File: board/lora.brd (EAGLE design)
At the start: 20.2 x 72.9 mm, 33 parts, among them IC1 STM32F030F4, IC2 ADP1607, J1 SWD_PTH_SHROUD, X1 SMA-142-0701-801/806, X2 UBLOX_MAX, X3 RFM98

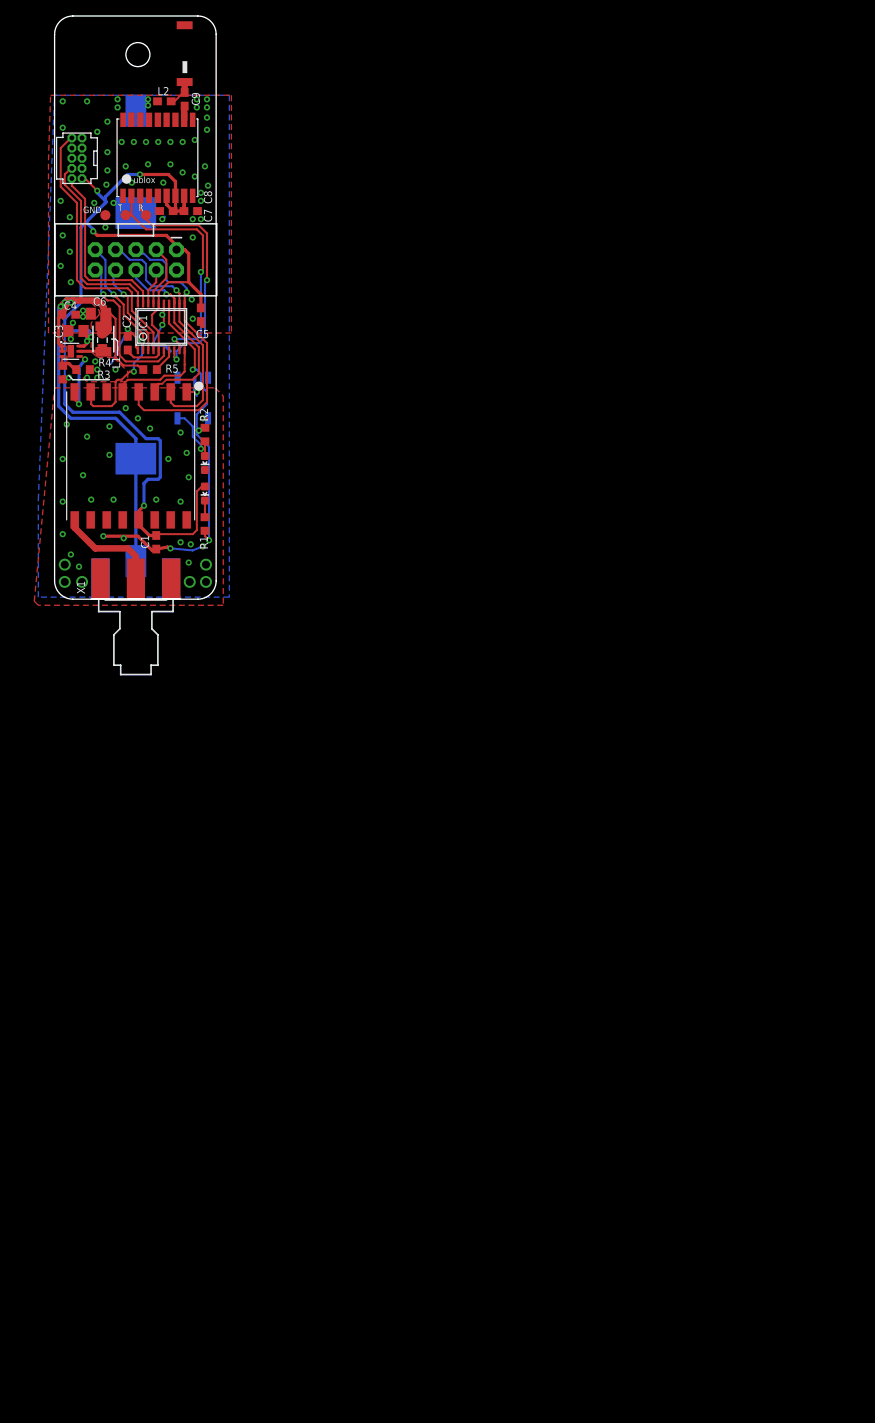
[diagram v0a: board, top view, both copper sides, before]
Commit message: improvments
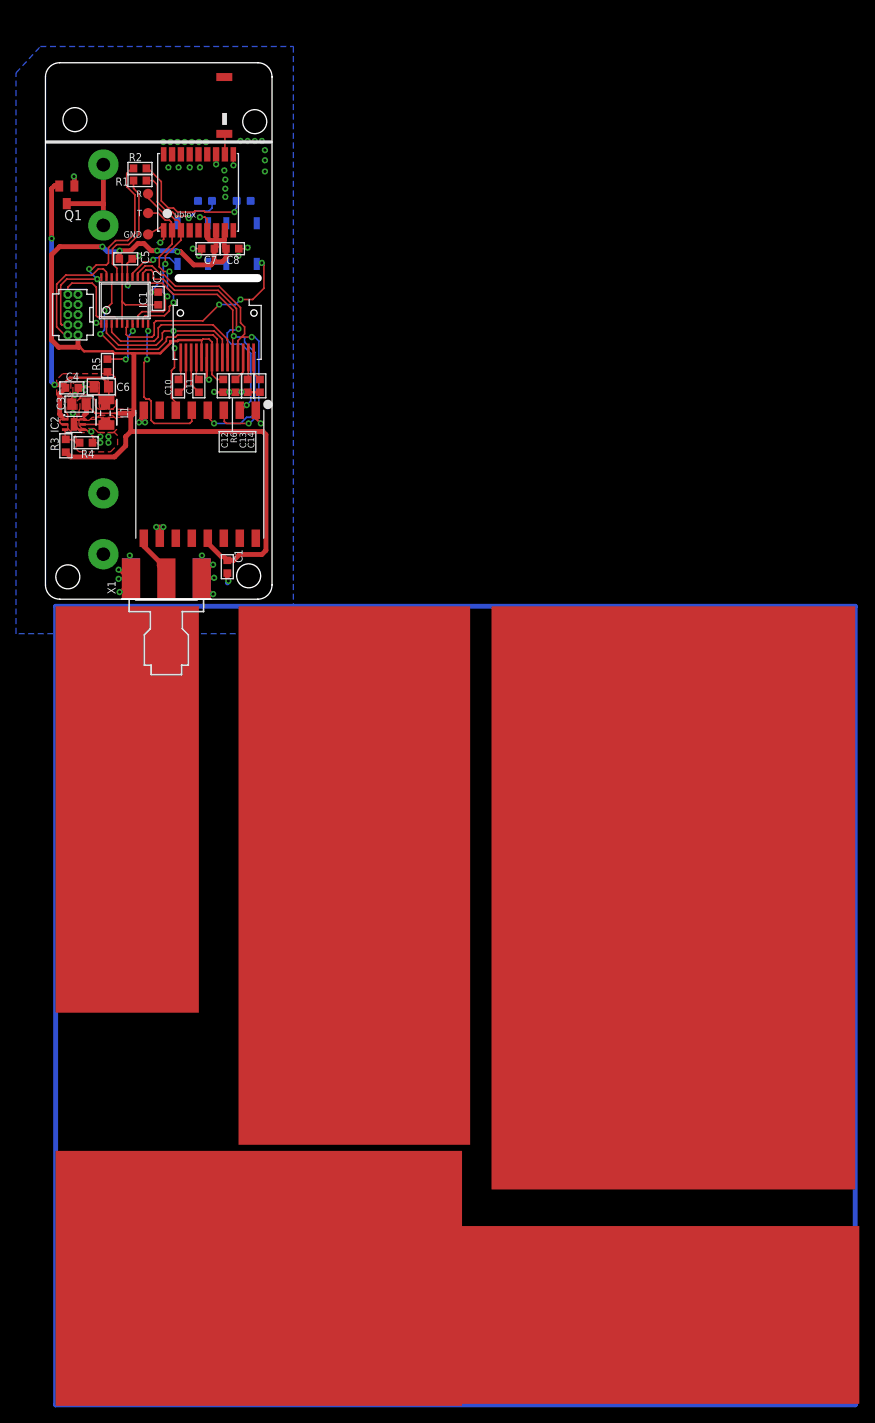
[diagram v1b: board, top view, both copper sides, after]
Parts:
- removed C9: (no value), rcl:C0603
- removed JP1: M05X2SHD, SparkFun-Connectors:2X5-SHROUDED
- removed L2: (no value), SparkFun-Passives:0603
- removed U$1: (no value), Mine:SUSF-XSM
- added C10, C11, C12: 1u, passives-7351:C0603-N
- added C13, C14: 2u2, passives-7351:C0603-N
- added Q1: BSS84, transistor-small-signal:SOT23
- added R6: 390k, passives-7351:R0603-N
- added S2: (no value), Mine:TACTILE_SWITCH_SMD
- added U$2: 091OLED, ukhas:0.91OLEDCON
- added U$3: (no value), ukhas:0.91OLEDPANEL
- C1, C2, C4, C5, C7, C8: device rcl:C0603 -> passives-7351:C0603-N
- C3, C6: device rcl:C0805 -> passives-7351:C0805-N
- R1, R2, R3, R4, R5: device rcl:R0603 -> passives-7351:R0603-N
- S1: value SWITCH-MOMENTARY-2SMD -> (none)
- U$6: value KEYSTONE-53 -> KEYSTONE-92; device Mine:KEYSTONE53 -> Mine:KEYSTONE-92-AA-BATTERY
- moved R1 43.7 mm to (10.7, 53.1), turned to 180 degrees
- moved LED1 36.6 mm to (18.8, 50.5), flipped to the bottom, turned to 270 degrees
- moved R2 34.3 mm to (10.7, 54.6), turned to 180 degrees
- moved LED2 33.1 mm to (23.6, 50.5), flipped to the bottom, turned to 90 degrees
- moved S1 20.2 mm to (23.4, 45.2)
- moved J1 19.6 mm to (2.29, 36.3)
- moved C5 11.7 mm to (8.89, 43.3), turned to 0 degrees
- moved C1 9.40 mm to (21.6, 4.83)
- moved C4 9.15 mm to (2.16, 27.2)
- moved L3 9.15 mm to (6.48, 24.1)
- moved C3 9.15 mm to (3.05, 25.1)
- moved C6 9.15 mm to (5.84, 27.3)
- moved IC2 9.15 mm to (2.41, 22.6)
- moved L1 9.15 mm to (6.35, 24.0)
- moved R3 9.15 mm to (1.40, 19.9)
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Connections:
- removed net GPIO1: IC1.3, JP1.8
- removed net GPIO3: IC1.6, JP1.10
- removed net N$10: X3.6
- removed net SCL: IC1.17, JP1.3
- removed net SDA: IC1.18, JP1.4
- new net D_C: IC1.3, U$2.10
- new net N$11: C10.2, U$2.1
- new net N$12: C11.2, U$2.3
- new net N$13: C11.1, U$2.4
- new net N$14: C10.1, U$2.2
- new net N$15: C13.1, U$2.14
- new net N$16: R6.2, U$2.13
- new net N$18: IC1.6, S1.1
- new net N$20: IC1.17, R1.2
- new net P_RST: IC1.2, U$2.9, X3.6
- new net S_CS: IC1.18, U$2.8
- new net VCC: C14.2, U$2.15
- net +3V3: now also C12.1, U$2.5, U$2.7; no longer JP1.1, LED1.A
- net GND: now also C12.2, C13.2, C14.1, LED1.C, Q1.1, R6.1, S1.3, S2.1, U$2.6, U$6.GND, U$6.GND2; no longer JP1.2, L2.2, S1.1, U$6.N1, U$6.N2
- net GPIO2: no longer IC1.2, JP1.9
- net MISO: no longer JP1.7
- net MOSI: now also U$2.12; no longer JP1.6
- net N$1: now also LED1.A, R1.1; no longer C9.2, X2.11_RF_IN
- net N$4: now also X2.11_RF_IN; no longer C9.1, L2.1
- net N$5: no longer S1.3
- net N$7: now also Q1.3, U$6.VBATT, U$6.VBATT1; no longer LED1.C, R1.2
- net N$8: now also S2.3; no longer R1.1, R2.2
- net SCLK: now also U$2.11; no longer JP1.5
- net SWCLK: now also R2.2
- net VBAT: now also Q1.2; no longer U$6.P1, U$6.P2
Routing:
- net N$10: track 0.00 -> 399.5 mm
- net GND: track 47.2 -> 78.2 mm, vias 101 -> 61
- net P_RST: track 0.00 -> 30.5 mm, vias 0 -> 2
- net GPIO2: track 29.8 -> 0.00 mm, vias 3 -> 0
- net N$8: track 36.7 -> 7.22 mm, vias 3 -> 1
- net VBAT: track 72.4 -> 45.2 mm, vias 3 -> 2
- net S_CS: track 0.00 -> 26.6 mm, vias 0 -> 2
- net N$18: track 0.00 -> 26.1 mm, vias 0 -> 3
- net RST: track 35.3 -> 11.8 mm
- net D_C: track 0.00 -> 20.5 mm
- net GPIO3: track 19.6 -> 0.00 mm, vias 1 -> 0
- net +3V3: track 144.8 -> 163.4 mm, vias 7 -> 5
- net MOSI: track 25.3 -> 40.5 mm, vias 1 -> 2
- net N$20: track 0.00 -> 14.8 mm
- net GPIO1: track 12.1 -> 0.00 mm, vias 1 -> 0
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- added copper zone on layer 1, net +3V3
- added copper zone on layer 1, net N$3
- added copper zone on layer 1, net VBAT
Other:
- board size 20.2 x 72.9 mm -> 28.3 x 67.1 mm
- board text added: "Err"
- board text added: "IC2"
- board text added: "Keep metal out of this area"
- board text added: "OK"
- board text removed: "Matt Brejza"
- board text removed: "Sept 14"
